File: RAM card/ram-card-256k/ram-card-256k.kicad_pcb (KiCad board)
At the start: 2 copper layers, 41.9 x 53.3 mm, 12 parts, among them J1 RAM card connector, U1 HC138, U2 KM681000BLG, U3 KM681000BLG

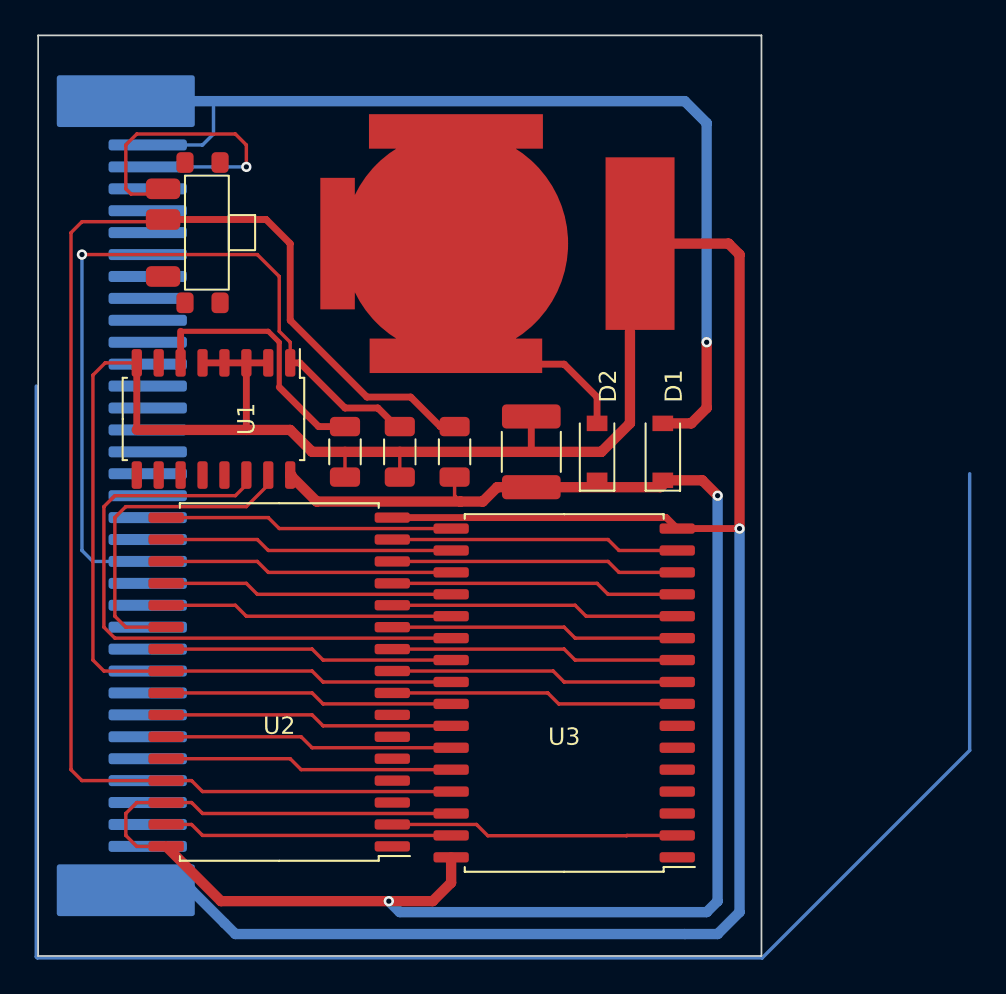
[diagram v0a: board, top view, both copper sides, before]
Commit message: Layout
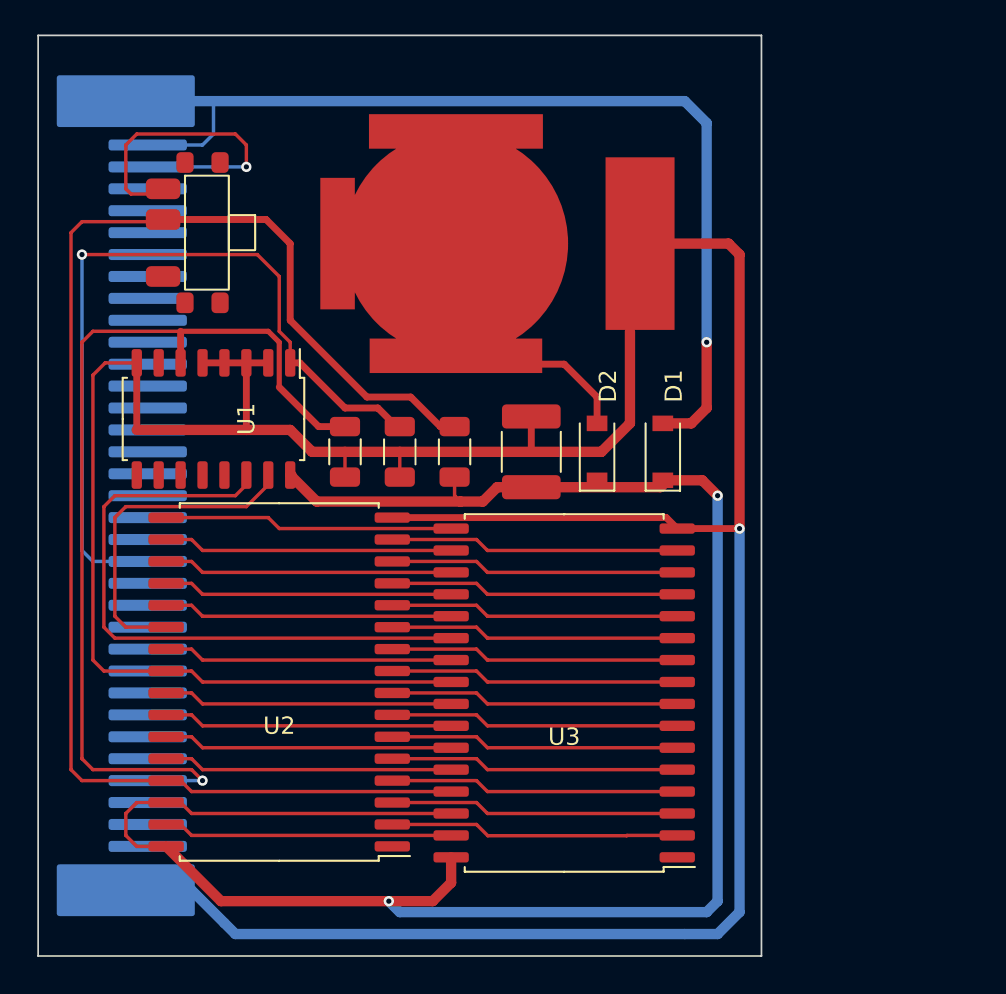
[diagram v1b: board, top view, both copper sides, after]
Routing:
- net (no net): track 108.2 -> 0.00 mm
- net Net-(J1-Pad31): track 15.1 -> 55.9 mm, vias 0 -> 1
- net /A6: track 0.00 -> 16.8 mm
- net /A14: track 0.00 -> 16.8 mm
- net /A12: track 0.00 -> 16.8 mm
- net /A5: track 0.00 -> 16.8 mm
- net /A7: track 0.00 -> 16.8 mm
